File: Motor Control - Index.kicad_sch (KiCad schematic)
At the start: 9 parts, among them J2 BM09B-SRSS-TB, U10 TB9051FTG,EL

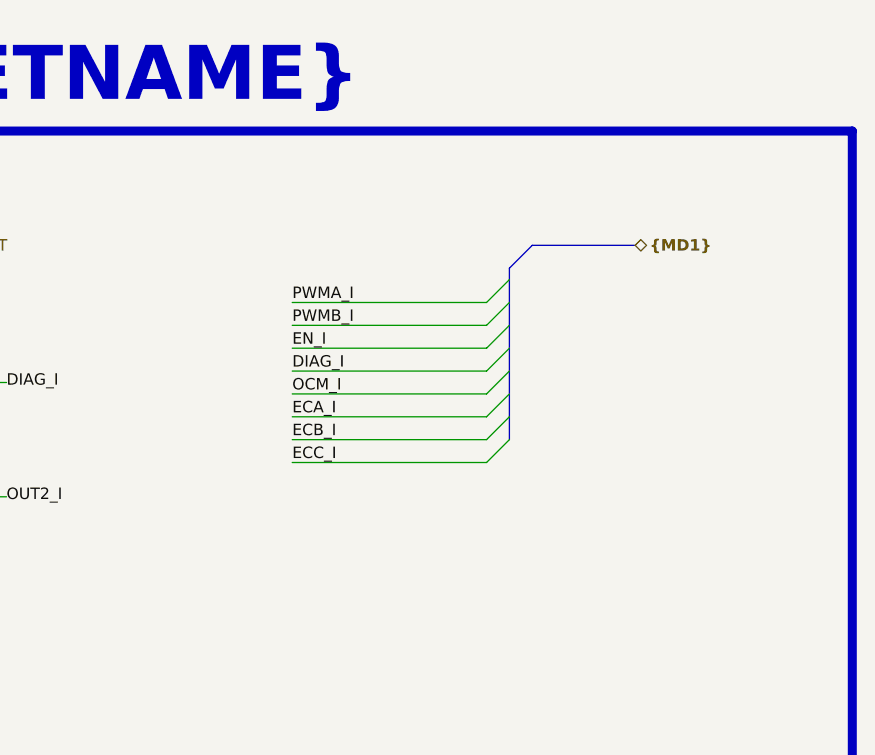
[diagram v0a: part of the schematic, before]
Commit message: Update Schematic
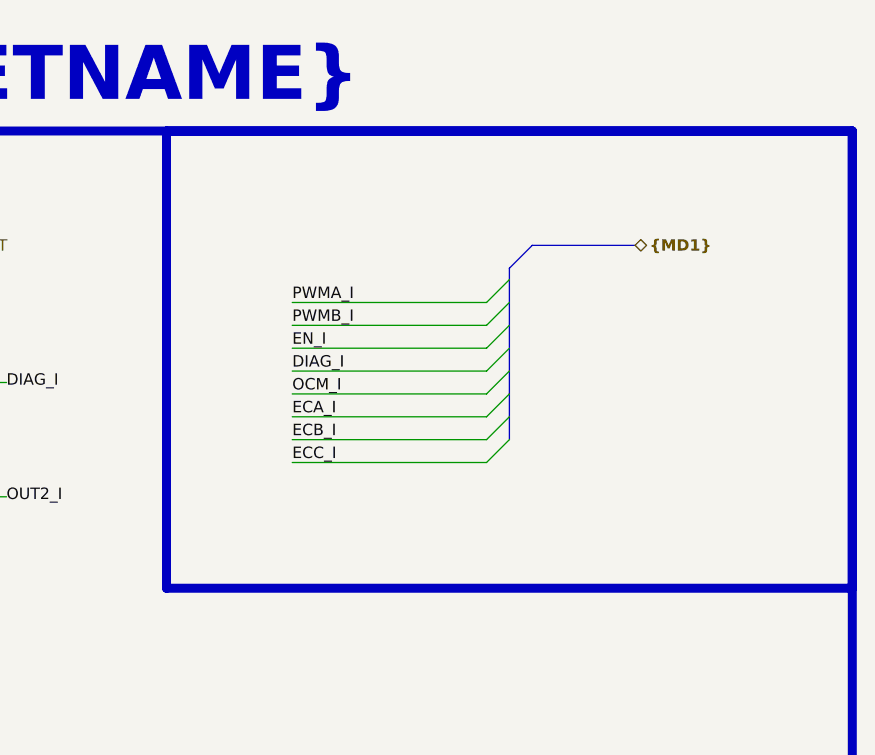
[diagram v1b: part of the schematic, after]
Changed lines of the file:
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@@
+	)
+	(rectangle
+		(start 177.8 25.4)
+		(end 254 76.2)
+		(stroke
+			(width 1)
+			(type default)
+			(color 200 0 0 1)
+		)
+		(fill
+			(type none)
+		)
 	)
 	(rectangle

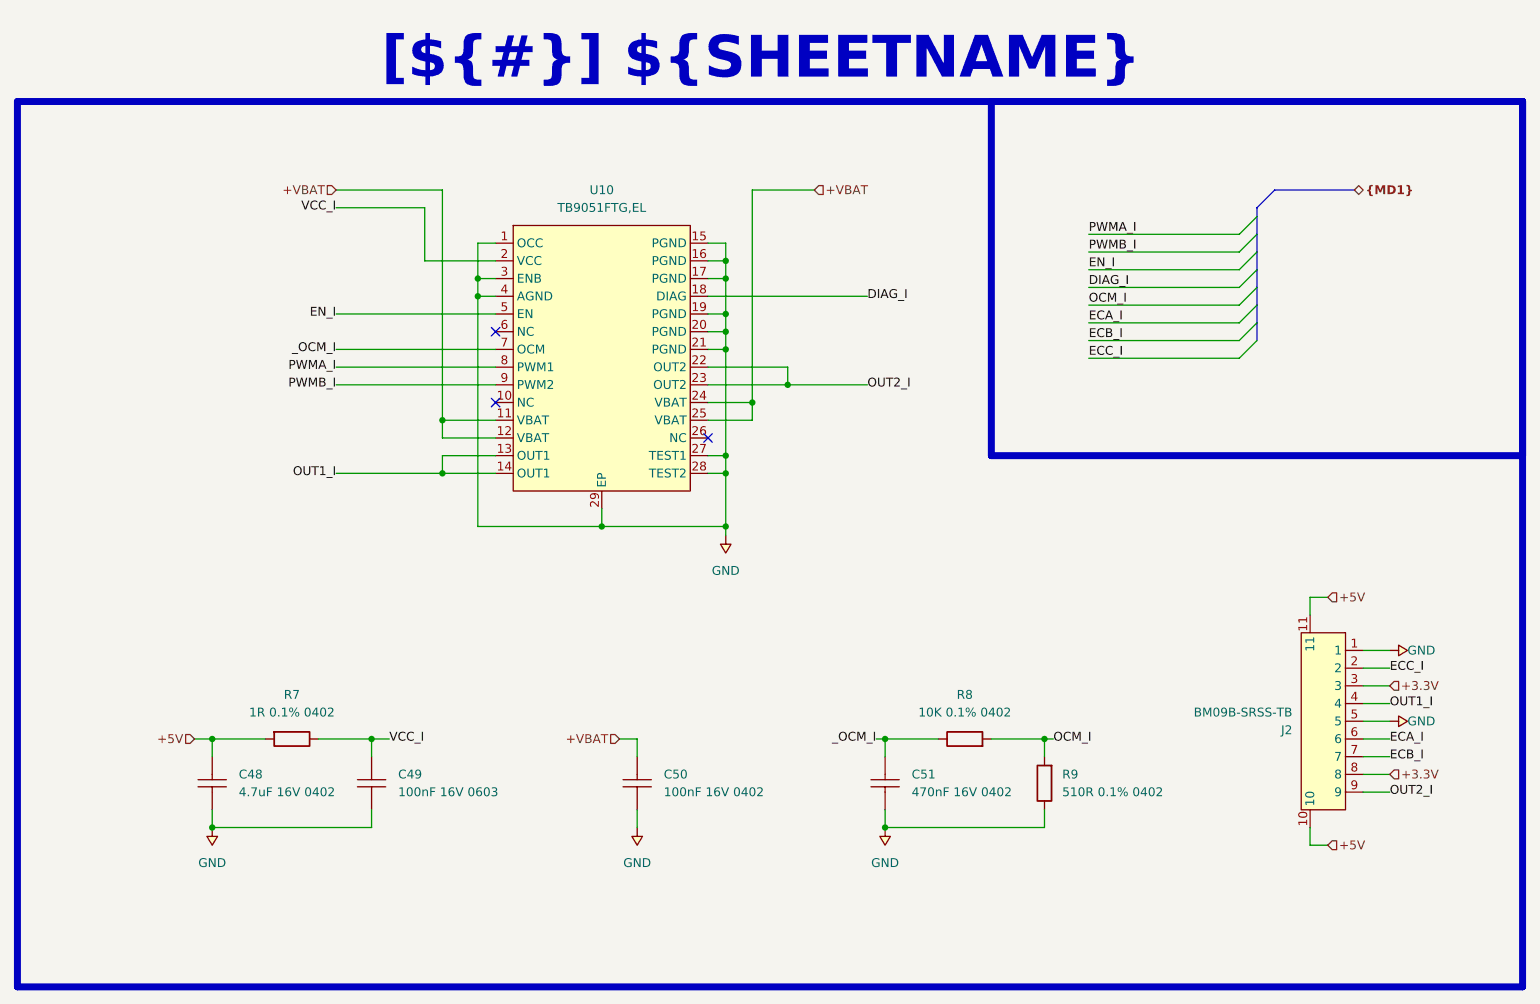
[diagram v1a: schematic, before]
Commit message: Update Schematic
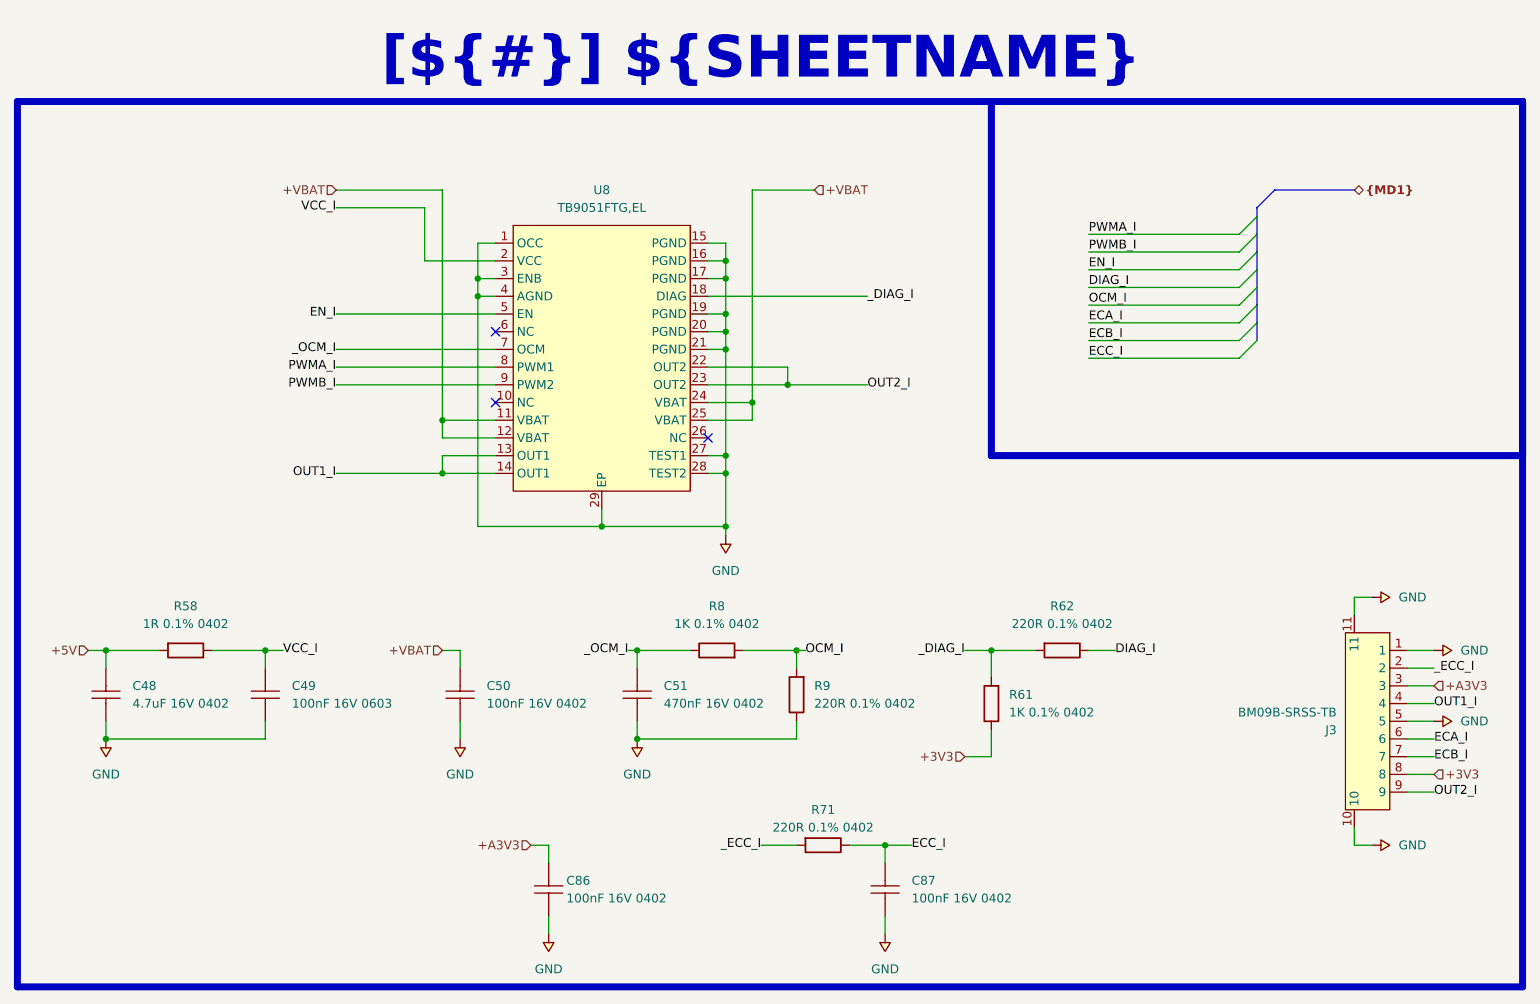
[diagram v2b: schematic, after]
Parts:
- removed R7: 1R 0.1% 0402, Duc_Library:R0402, symbol Duc-Resistors:RES SMD 0402
- added C86, C87: 100nF 16V 0402, Duc_Library:C0402, symbol Duc-Capacitors:CAP CER 0402
- added R58: 1R 0.1% 0402, Duc_Library:R0402, symbol Duc-Resistors:RES SMD 0402
- added R61: 1K 0.1% 0402, Duc_Library:R0402, symbol Duc-Resistors:RES SMD 0402
- added R62, R71: 220R 0.1% 0402, Duc_Library:R0402, symbol Duc-Resistors:RES SMD 0402
- R8: value 10K 0.1% 0402 -> 1K 0.1% 0402
- R9: value 510R 0.1% 0402 -> 220R 0.1% 0402
- renumbered J2 to J3, U10 to U8
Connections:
- net +5V: now also R58.1; no longer J3.10, J3.11
- net DIAG_I: now also R62.2; no longer U8.18 (DIAG)
- net ECC_I: now also C87.2, R71.2; no longer J3.2
- net GND: now also J3.10, J3.11, C86.1, C87.1
- net VCC_I: now also R58.2
- net +3.3V renamed +3V3
- net +3V3: now also R61.2; no longer J3.3
- new net +A3V3: C86.2, J3.3
- new net _DIAG_I: R61.1, R62.1, U8.18 (DIAG)
- new net _ECC_I: J3.2, R71.1
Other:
- moved on the sheet: C48, C49, C50, C51, J3, R8, R9
